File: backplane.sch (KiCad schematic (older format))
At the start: 15 parts, among them J1 I2C_HEADER, J2 GPS_HEADER, J3 SERIAL_HEADER, J4 PWR_HEADER, Q1 Q_NMOS_DGS, Q2 Q_NMOS_DGS, Q3 Q_NMOS_DGS, U1 Raspberry_Pi_2_3, U2 IC880A-SPI

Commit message: Remove GPS header (fixes #1)
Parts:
- removed J2: GPS_HEADER, Pin_Headers:Pin_Header_Straight_1x06_Pitch2.54mm, symbol GPS_HEADER
- R1, R2, R3: symbol R -> R-RESCUE-backplane
- U2: footprint ic880a:IC880A-SPI -> (none)
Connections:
- wire segments 120 -> 105
- no-connect marks 23 -> 26
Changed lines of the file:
@@
 EESchema Schematic File Version 2
+LIBS:backplane-rescue
 LIBS:power
 LIBS:device
@@
 $EndComp
 $Comp
-L GPS_HEADER J2
-U 1 1 58960C52
-P 10350 1400
-F 0 "J2" H 10350 1000 60  0000 C CNN
-F 1 "GPS_HEADER" H 10350 1800 60  0000 C CNN
-F 2 "Pin_Headers:Pin_Header_Straight_1x06_Pitch2.54mm" H 10350 1450 60  0001 C CNN
-F 3 "" H 10350 1450 60  0001 C CNN
-	1    10350 1400
-	1    0    0    -1
-$EndComp
-$Comp
 L SERIAL_HEADER J3
 U 1 1 58961502
@@
 $EndComp
 $Comp
-L IC880A-SPI U2
-U 3 1 589605EF
-P 8450 1600
-F 0 "U2" H 8450 1000 60  0000 C CNN
-F 1 "IC880A-SPI" H 8450 2200 60  0000 C CNN
-F 2 "ic880a:IC880A-SPI" H 8450 1600 60  0001 C CNN
-F 3 "" H 8450 1600 60  0001 C CNN
-	3    8450 1600
-	1    0    0    -1
-$EndComp
-$Comp
-L R R3
+L R-RESCUE-backplane R3
 U 1 1 58964C66
 P 1500 2650
@@
 $EndComp
 $Comp
-L R R2
+L R-RESCUE-backplane R2
 U 1 1 58965066
 P 1200 2650
@@
 $EndComp
 $Comp
-L R R1
+L R-RESCUE-backplane R1
 U 1 1 589650B2
 P 900 2650
@@
 $EndComp
 $Comp
-L GND #PWR01
+L GND-RESCUE-backplane #PWR1
 U 1 1 58965F26
 P 2850 3600
-F 0 "#PWR01" H 2850 3350 50  0001 C CNN
+F 0 "#PWR1" H 2850 3350 50  0001 C CNN
 F 1 "GND" H 2850 3450 50  0000 C CNN
 F 2 "" H 2850 3600 50  0000 C CNN
@@
 $EndComp
 $Comp
-L GND #PWR02
+L GND-RESCUE-backplane #PWR2
 U 1 1 58965F7C
 P 2850 4150
-F 0 "#PWR02" H 2850 3900 50  0001 C CNN
+F 0 "#PWR2" H 2850 3900 50  0001 C CNN
 F 1 "GND" H 2850 4000 50  0000 C CNN
 F 2 "" H 2850 4150 50  0000 C CNN
@@
 $EndComp
 $Comp
-L GND #PWR03
+L GND-RESCUE-backplane #PWR3
 U 1 1 58965FBA
 P 2850 4700
-F 0 "#PWR03" H 2850 4450 50  0001 C CNN
+F 0 "#PWR3" H 2850 4450 50  0001 C CNN
 F 1 "GND" H 2850 4550 50  0000 C CNN
 F 2 "" H 2850 4700 50  0000 C CNN
@@
 	1    0    0    -1
 $EndComp
-$Comp
-L PWR_FLAG #FLG04
-U 1 1 58968B52
-P 9650 1700
-F 0 "#FLG04" H 9650 1795 50  0001 C CNN
-F 1 "PWR_FLAG" H 9650 1880 50  0000 C CNN
-F 2 "" H 9650 1700 50  0000 C CNN
-F 3 "" H 9650 1700 50  0000 C CNN
-	1    9650 1700
-	-1   0    0    1
-$EndComp
 Wire Wire Line
 	4850 1550 4850 3200
@@
 	4950 2600 4950 3200
 Wire Wire Line
-	9150 1150 9950 1150
-Wire Wire Line
-	9950 1250 9150 1250
-Wire Wire Line
-	9150 1350 9950 1350
-Wire Wire Line
-	9950 1450 9300 1450
-Wire Wire Line
-	9300 1450 9300 2800
-Wire Wire Line
-	9300 2800 5250 2800
-Wire Wire Line
 	5250 2800 5250 3200
-Wire Wire Line
-	9950 1550 9400 1550
-Wire Wire Line
-	9400 1550 9400 2900
-Wire Wire Line
-	9400 2900 4950 2900
 Connection ~ 4950 2900
-Wire Wire Line
-	9950 1650 9900 1650
-Wire Wire Line
-	9900 1650 9900 2000
-Wire Wire Line
-	9900 2000 10800 2000
-Wire Wire Line
-	10800 2000 10800 900
-Wire Wire Line
-	10800 900  4400 900
-Wire Wire Line
-	4400 900  4400 2000
-Wire Wire Line
-	4400 2000 4250 2000
 Wire Wire Line
 	5950 5200 6050 5200
@@
 Connection ~ 2850 4150
 Wire Wire Line
-	9650 1700 9650 1350
-Connection ~ 9650 1350
-Wire Wire Line
 	2500 3600 2850 3600
 $Comp
-L GND #PWR05
+L GND-RESCUE-backplane #PWR4
 U 1 1 5896BA26
 P 4350 6200
-F 0 "#PWR05" H 4350 5950 50  0001 C CNN
+F 0 "#PWR4" H 4350 5950 50  0001 C CNN
 F 1 "GND" H 4350 6050 50  0000 C CNN
 F 2 "" H 4350 6200 50  0000 C CNN
@@
 	9000 3500 9000 3600
 $Comp
-L GND #PWR06
+L GND-RESCUE-backplane #PWR7
 U 1 1 589714DC
 P 9000 3600
-F 0 "#PWR06" H 9000 3350 50  0001 C CNN
+F 0 "#PWR7" H 9000 3350 50  0001 C CNN
 F 1 "GND" H 9000 3450 50  0000 C CNN
 F 2 "" H 9000 3600 50  0000 C CNN
@@
 	8350 4550 8350 4600
 $Comp
-L GND #PWR07
+L GND-RESCUE-backplane #PWR6
 U 1 1 589715AD
 P 8350 4600
-F 0 "#PWR07" H 8350 4350 50  0001 C CNN
+F 0 "#PWR6" H 8350 4350 50  0001 C CNN
 F 1 "GND" H 8350 4450 50  0000 C CNN
 F 2 "" H 8350 4600 50  0000 C CNN
@@
 	6800 3350 6800 3450
 $Comp
-L GND #PWR08
+L GND-RESCUE-backplane #PWR5
 U 1 1 589716C7
 P 6800 3450
-F 0 "#PWR08" H 6800 3200 50  0001 C CNN
+F 0 "#PWR5" H 6800 3200 50  0001 C CNN
 F 1 "GND" H 6800 3300 50  0000 C CNN
 F 2 "" H 6800 3450 50  0000 C CNN
@@
 3.3V
 NoConn ~ 4650 5800
+NoConn ~ 4250 2000
+$Comp
+L IC880A-SPI U2
+U 3 1 5898B4F6
+P 10000 1400
+F 0 "U2" H 10000 800 60  0000 C CNN
+F 1 "IC880A-SPI" H 10000 2000 60  0000 C CNN
+F 2 "" H 10000 1400 60  0001 C CNN
+F 3 "" H 10000 1400 60  0001 C CNN
+	3    10000 1400
+	1    0    0    -1
+$EndComp
+Wire Wire Line
+	10700 1150 10750 1150
+Wire Wire Line
+	10750 1150 10750 1200
+$Comp
+L GND #PWR8
+U 1 1 5898B674
+P 10750 1200
+F 0 "#PWR8" H 10750 1200 30  0001 C CNN
+F 1 "GND" H 10750 1130 30  0001 C CNN
+F 2 "" H 10750 1200 60  0001 C CNN
+F 3 "" H 10750 1200 60  0001 C CNN
+	1    10750 1200
+	1    0    0    -1
+$EndComp
+NoConn ~ 10700 950
+NoConn ~ 10700 1050
 $EndSCHEMATC

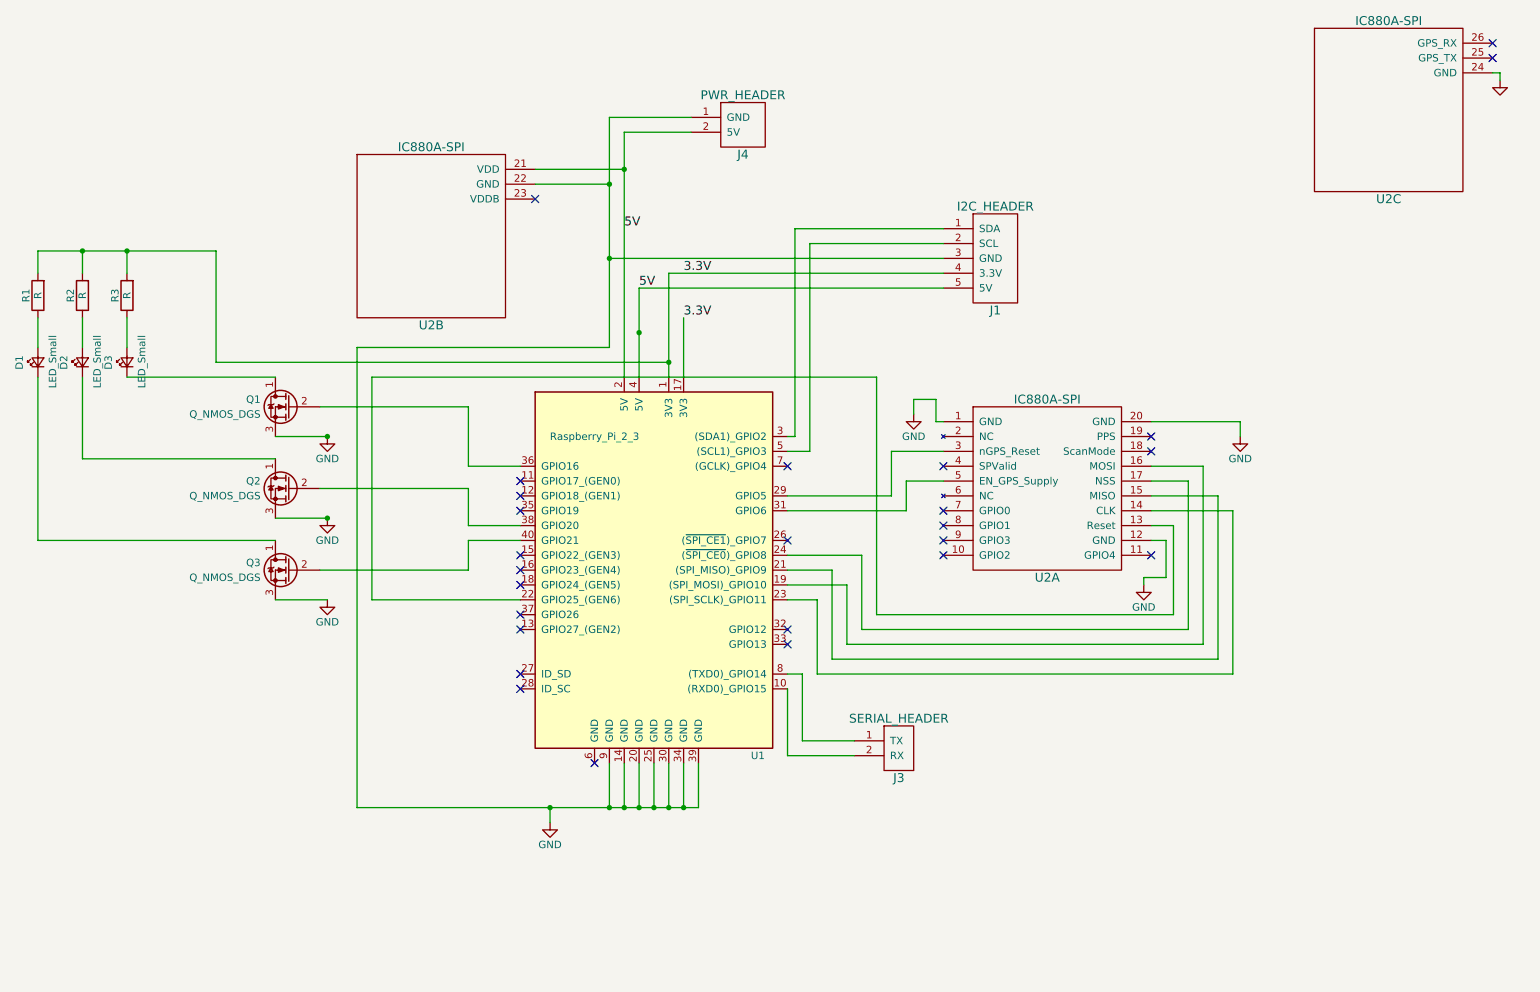
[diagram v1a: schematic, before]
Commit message: Add SHT21 to schema
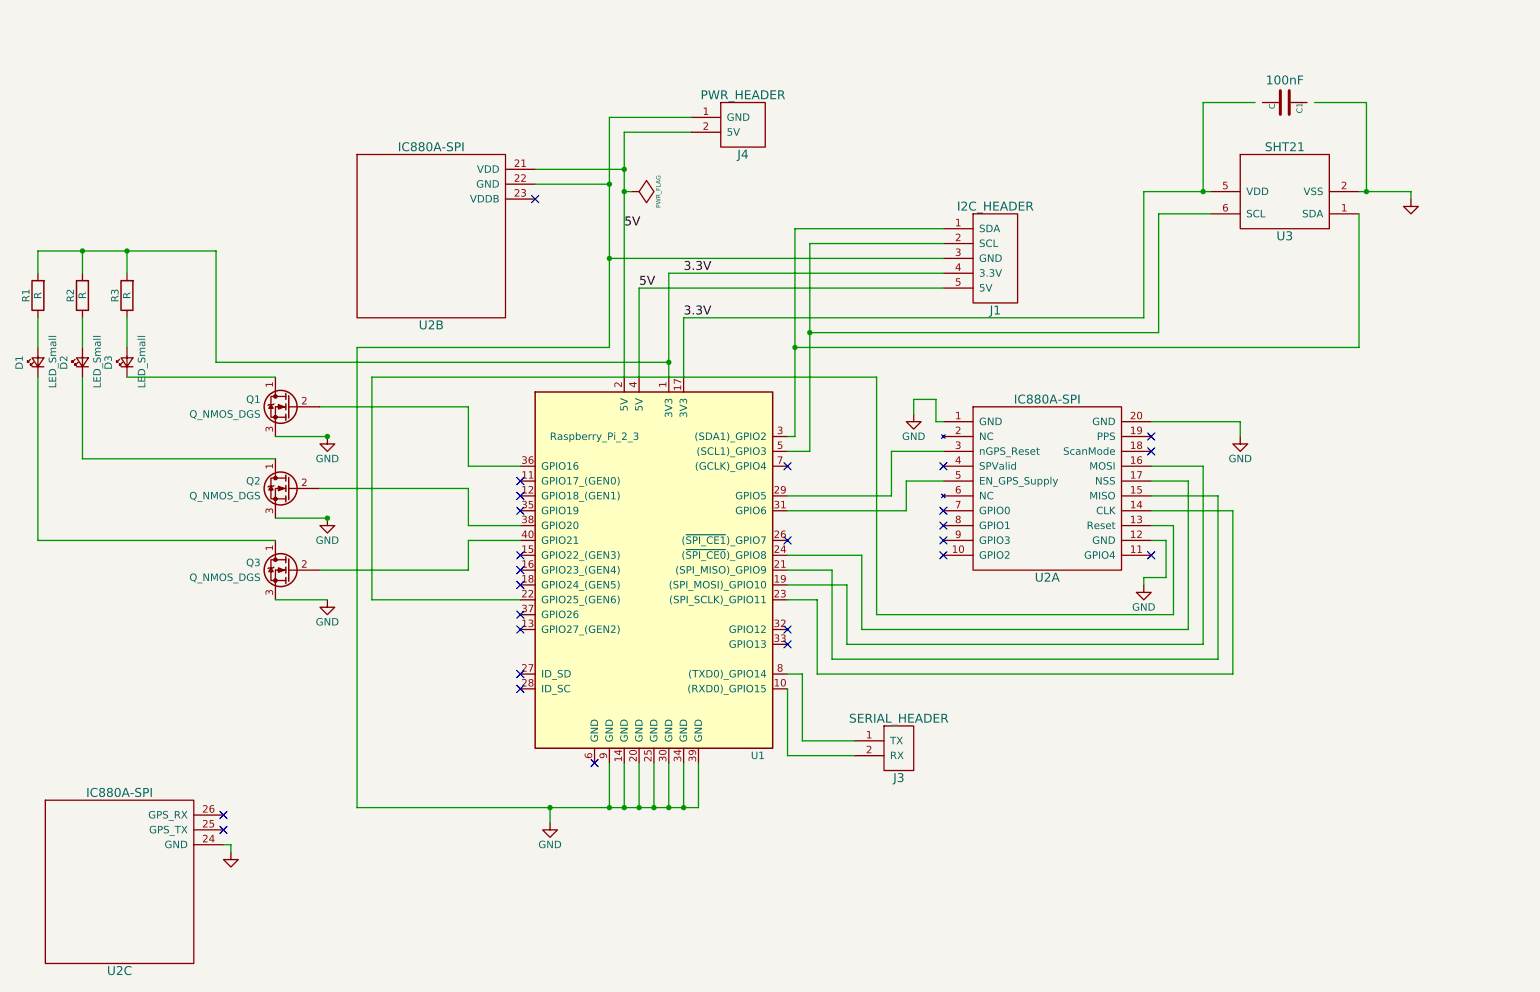
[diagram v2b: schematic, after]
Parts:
- added C1: C, symbol C
- added U3: SHT21, symbol SHT21
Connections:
- net 3.3V: now also U3.5 (VDD)
- net GND: now also U3.2 (VSS)
- net at J1.1 (SDA), U1.3 ((SDA1)_GPIO2): now also U3.1 (SDA)
- net at J1.2 (SCL), U1.5 ((SCL1)_GPIO3): now also U3.6 (SCL)
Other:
- moved on the sheet: U2C
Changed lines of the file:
@@
 EESchema Schematic File Version 2
-LIBS:backplane-rescue
 LIBS:power
 LIBS:device
@@
 LIBS:headers
 LIBS:raspi
+LIBS:sensirion
 LIBS:backplane-cache
 EELAYER 25 0
@@
 $EndComp
 $Comp
-L GND-RESCUE-backplane #PWR1
+L GND-RESCUE-backplane #PWR01
 U 1 1 58965F26
 P 2850 3600
-F 0 "#PWR1" H 2850 3350 50  0001 C CNN
+F 0 "#PWR01" H 2850 3350 50  0001 C CNN
 F 1 "GND" H 2850 3450 50  0000 C CNN
 F 2 "" H 2850 3600 50  0000 C CNN
@@
 $EndComp
 $Comp
-L GND-RESCUE-backplane #PWR2
+L GND-RESCUE-backplane #PWR02
 U 1 1 58965F7C
 P 2850 4150
-F 0 "#PWR2" H 2850 3900 50  0001 C CNN
+F 0 "#PWR02" H 2850 3900 50  0001 C CNN
 F 1 "GND" H 2850 4000 50  0000 C CNN
 F 2 "" H 2850 4150 50  0000 C CNN
@@
 $EndComp
 $Comp
-L GND-RESCUE-backplane #PWR3
+L GND-RESCUE-backplane #PWR03
 U 1 1 58965FBA
 P 2850 4700
-F 0 "#PWR3" H 2850 4450 50  0001 C CNN
+F 0 "#PWR03" H 2850 4450 50  0001 C CNN
 F 1 "GND" H 2850 4550 50  0000 C CNN
 F 2 "" H 2850 4700 50  0000 C CNN
@@
 	8550 4200 8400 4200
 Wire Wire Line
-	5950 3600 6000 3600
-Wire Wire Line
-	6000 3600 6000 2200
+	6000 3600 5950 3600
+Wire Wire Line
+	6000 2200 6000 3600
 Wire Wire Line
 	6000 2200 7000 2200
@@
 Wire Wire Line
 	5250 2800 5250 3200
-Connection ~ 4950 2900
 Wire Wire Line
 	5950 5200 6050 5200
@@
 	2500 3600 2850 3600
 $Comp
-L GND-RESCUE-backplane #PWR4
+L GND-RESCUE-backplane #PWR04
 U 1 1 5896BA26
 P 4350 6200
-F 0 "#PWR4" H 4350 5950 50  0001 C CNN
+F 0 "#PWR04" H 4350 5950 50  0001 C CNN
 F 1 "GND" H 4350 6050 50  0000 C CNN
 F 2 "" H 4350 6200 50  0000 C CNN
@@
 	9000 3500 9000 3600
 $Comp
-L GND-RESCUE-backplane #PWR7
+L GND-RESCUE-backplane #PWR05
 U 1 1 589714DC
 P 9000 3600
-F 0 "#PWR7" H 9000 3350 50  0001 C CNN
+F 0 "#PWR05" H 9000 3350 50  0001 C CNN
 F 1 "GND" H 9000 3450 50  0000 C CNN
 F 2 "" H 9000 3600 50  0000 C CNN
@@
 	8350 4550 8350 4600
 $Comp
-L GND-RESCUE-backplane #PWR6
+L GND-RESCUE-backplane #PWR06
 U 1 1 589715AD
 P 8350 4600
-F 0 "#PWR6" H 8350 4350 50  0001 C CNN
+F 0 "#PWR06" H 8350 4350 50  0001 C CNN
 F 1 "GND" H 8350 4450 50  0000 C CNN
 F 2 "" H 8350 4600 50  0000 C CNN
@@
 	6800 3350 6800 3450
 $Comp
-L GND-RESCUE-backplane #PWR5
+L GND-RESCUE-backplane #PWR07
 U 1 1 589716C7
 P 6800 3450
-F 0 "#PWR5" H 6800 3200 50  0001 C CNN
+F 0 "#PWR07" H 6800 3200 50  0001 C CNN
 F 1 "GND" H 6800 3300 50  0000 C CNN
 F 2 "" H 6800 3450 50  0000 C CNN
@@
 L IC880A-SPI U2
 U 3 1 5898B4F6
-P 10000 1400
-F 0 "U2" H 10000 800 60  0000 C CNN
-F 1 "IC880A-SPI" H 10000 2000 60  0000 C CNN
-F 2 "" H 10000 1400 60  0001 C CNN
-F 3 "" H 10000 1400 60  0001 C CNN
-	3    10000 1400
-	1    0    0    -1
-$EndComp
-Wire Wire Line
-	10700 1150 10750 1150
-Wire Wire Line
-	10750 1150 10750 1200
-$Comp
-L GND #PWR8
+P 1450 6600
+F 0 "U2" H 1450 6000 60  0000 C CNN
+F 1 "IC880A-SPI" H 1450 7200 60  0000 C CNN
+F 2 "" H 1450 6600 60  0001 C CNN
+F 3 "" H 1450 6600 60  0001 C CNN
+	3    1450 6600
+	1    0    0    -1
+$EndComp
+Wire Wire Line
+	2150 6350 2200 6350
+Wire Wire Line
+	2200 6350 2200 6400
+$Comp
+L GND #PWR08
 U 1 1 5898B674
-P 10750 1200
-F 0 "#PWR8" H 10750 1200 30  0001 C CNN
-F 1 "GND" H 10750 1130 30  0001 C CNN
-F 2 "" H 10750 1200 60  0001 C CNN
-F 3 "" H 10750 1200 60  0001 C CNN
-	1    10750 1200
-	1    0    0    -1
-$EndComp
-NoConn ~ 10700 950
-NoConn ~ 10700 1050
+P 2200 6400
+F 0 "#PWR08" H 2200 6400 30  0001 C CNN
+F 1 "GND" H 2200 6330 30  0001 C CNN
+F 2 "" H 2200 6400 60  0001 C CNN
+F 3 "" H 2200 6400 60  0001 C CNN
+	1    2200 6400
+	1    0    0    -1
+$EndComp
+NoConn ~ 2150 6150
+NoConn ~ 2150 6250
+$Comp
+L SHT21 U3
+U 1 1 5898B996
+P 9300 1950
+F 0 "U3" H 9300 1650 60  0000 C CNN
+F 1 "SHT21" H 9300 2250 60  0000 C CNN
+F 2 "" H 9300 1950 60  0001 C CNN
+F 3 "" H 9300 1950 60  0001 C CNN
+	1    9300 1950
+	1    0    0    -1
+$EndComp
+Wire Wire Line
+	5250 2800 8350 2800
+Wire Wire Line
+	8350 2800 8350 1950
+Wire Wire Line
+	8350 1950 8800 1950
+Wire Wire Line
+	9800 1950 10150 1950
+Wire Wire Line
+	10150 1950 10150 2000
+$Comp
+L GND #PWR09
+U 1 1 5898C07A
+P 10150 2000
+F 0 "#PWR09" H 10150 2000 30  0001 C CNN
+F 1 "GND" H 10150 1930 30  0001 C CNN
+F 2 "" H 10150 2000 60  0001 C CNN
+F 3 "" H 10150 2000 60  0001 C CNN
+	1    10150 2000
+	1    0    0    -1
+$EndComp
+Wire Wire Line
+	6100 2900 8450 2900
+Wire Wire Line
+	8450 2900 8450 2100
+Wire Wire Line
+	8450 2100 8800 2100
+Connection ~ 6100 2900
+Wire Wire Line
+	6000 3000 9800 3000
+Wire Wire Line
+	9800 3000 9800 2100
+Connection ~ 6000 3000
+$Comp
+L C C1
+U 1 1 5898C4BA
+P 9300 1350
+F 0 "C1" H 9300 1450 40  0000 L CNN
+F 1 "C" H 9306 1265 40  0000 L CNN
+F 2 "" H 9338 1200 30  0000 C CNN
+F 3 "https://www.sensirion.com/fileadmin/user_upload/customers/sensirion/Dokumente/2_Humidity_Sensors/Sensirion_Humidity_Sensors_SHT21_Datasheet_V4.pdf" H 9300 1350 60  0001 C CNN
+F 4 "100nF" V 9150 1350 60  0000 C CNN "C"
+	1    9300 1350
+	0    1    1    0
+$EndComp
+Wire Wire Line
+	9850 1950 9850 1350
+Wire Wire Line
+	9850 1350 9500 1350
+Connection ~ 9850 1950
+Wire Wire Line
+	9100 1350 8750 1350
+Wire Wire Line
+	8750 1350 8750 1950
+Connection ~ 8750 1950
+$Comp
+L PWR_FLAG #FLG010
+U 1 1 5898DCF1
+P 4900 1950
+F 0 "#FLG010" H 4900 2045 30  0001 C CNN
+F 1 "PWR_FLAG" H 4900 2130 30  0000 C CNN
+F 2 "" H 4900 1950 60  0001 C CNN
+F 3 "" H 4900 1950 60  0001 C CNN
+	1    4900 1950
+	0    1    1    0
+$EndComp
+Wire Wire Line
+	4900 1950 4850 1950
+Connection ~ 4850 1950
 $EndSCHEMATC

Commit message: Add SHT21 sensor
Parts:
- C1: footprint (none) -> Capacitors_SMD:C_1206_HandSoldering
- U2: footprint (none) -> ic880a:IC880A-SPI
- U3: footprint (none) -> sensirion:SHT21
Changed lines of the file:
@@
 F 0 "U2" H 1450 6000 60  0000 C CNN
 F 1 "IC880A-SPI" H 1450 7200 60  0000 C CNN
-F 2 "" H 1450 6600 60  0001 C CNN
+F 2 "ic880a:IC880A-SPI" H 1450 6600 60  0001 C CNN
 F 3 "" H 1450 6600 60  0001 C CNN
 	3    1450 6600
@@
 F 0 "U3" H 9300 1650 60  0000 C CNN
 F 1 "SHT21" H 9300 2250 60  0000 C CNN
-F 2 "" H 9300 1950 60  0001 C CNN
+F 2 "sensirion:SHT21" H 9300 1950 60  0001 C CNN
 F 3 "" H 9300 1950 60  0001 C CNN
 	1    9300 1950
@@
 F 0 "C1" H 9300 1450 40  0000 L CNN
 F 1 "C" H 9306 1265 40  0000 L CNN
-F 2 "" H 9338 1200 30  0000 C CNN
+F 2 "Capacitors_SMD:C_1206_HandSoldering" H 9338 1200 30  0001 C CNN
 F 3 "https://www.sensirion.com/fileadmin/user_upload/customers/sensirion/Dokumente/2_Humidity_Sensors/Sensirion_Humidity_Sensors_SHT21_Datasheet_V4.pdf" H 9300 1350 60  0001 C CNN
 F 4 "100nF" V 9150 1350 60  0000 C CNN "C"
